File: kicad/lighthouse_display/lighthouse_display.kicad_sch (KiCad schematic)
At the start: 28 parts, among them J1 Conn_01x12_Pin, U1 IS31FL3731-SA, U2 TPS61176RTER

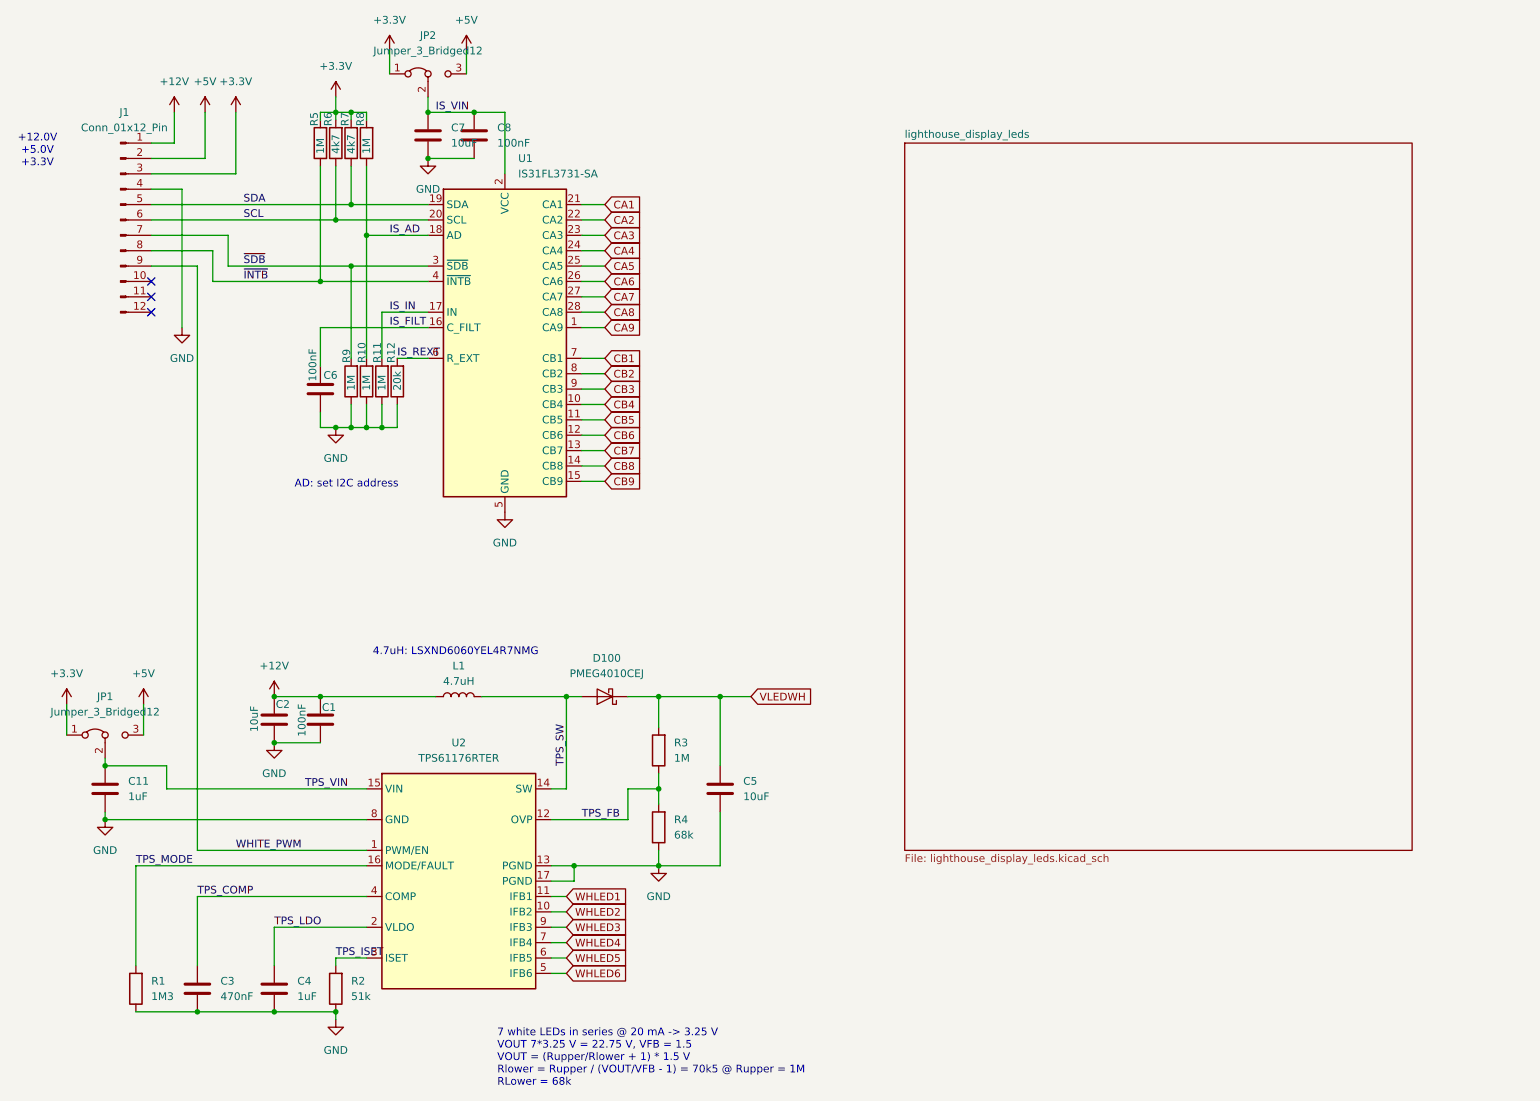
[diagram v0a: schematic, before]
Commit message: hardware for lighthouse display rev1 and button rev1 done
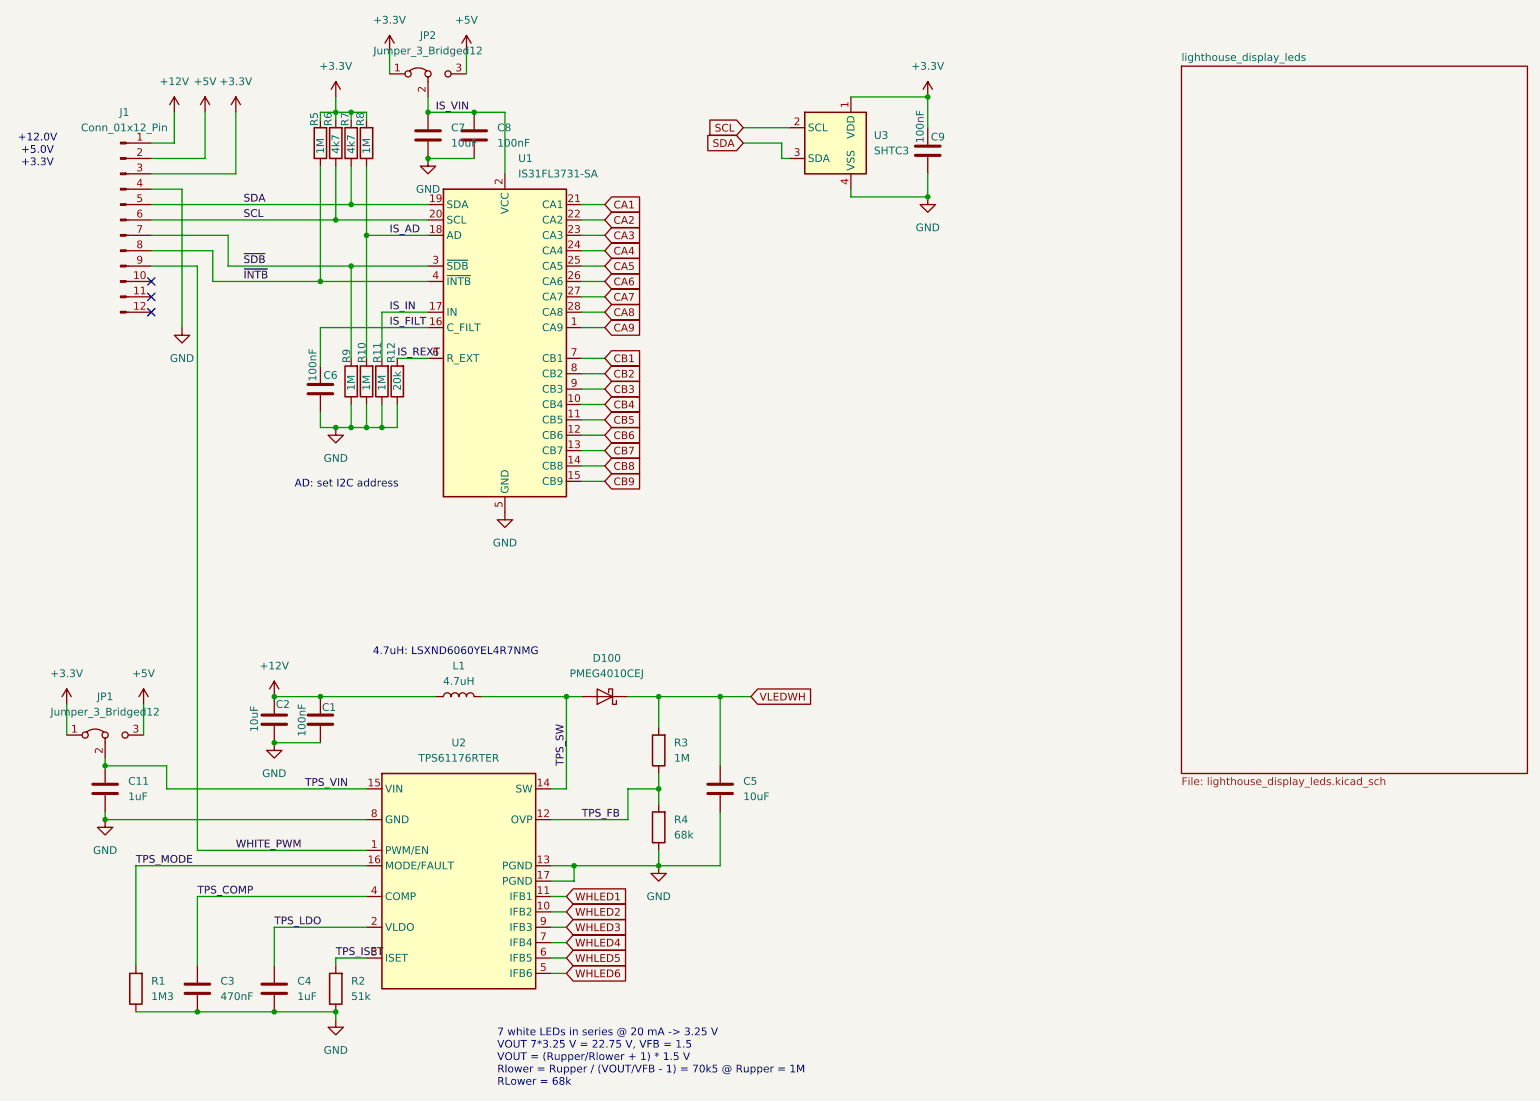
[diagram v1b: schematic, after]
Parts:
- added C9: 100nF, Capacitor_SMD:C_0603_1608Metric_Pad1.08x0.95mm_HandSolder, symbol Device:C
- added U3: SHTC3, Sensor_Humidity:Sensirion_DFN-4-1EP_2x2mm_P1mm_EP0.7x1.6mm, symbol Sensor_Humidity:SHTC3
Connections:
- net +3.3V: now also C9.1, U3.1 (VDD)
- net GND: now also C9.2, U3.4 (VSS)
- net SCL: now also U3.2 (SCL)
- net SDA: now also U3.3 (SDA)
